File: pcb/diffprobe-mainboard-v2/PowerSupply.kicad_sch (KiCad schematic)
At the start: 19 parts, among them J54 AC_P, J55 AC_N, J56 AC_E

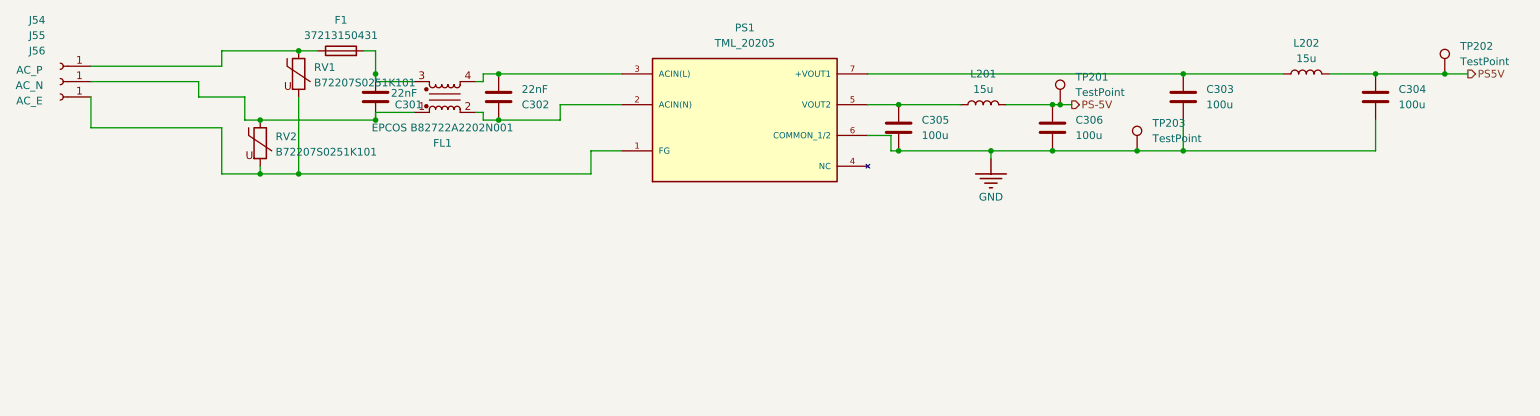
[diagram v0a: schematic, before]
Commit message: schematic cleanup again
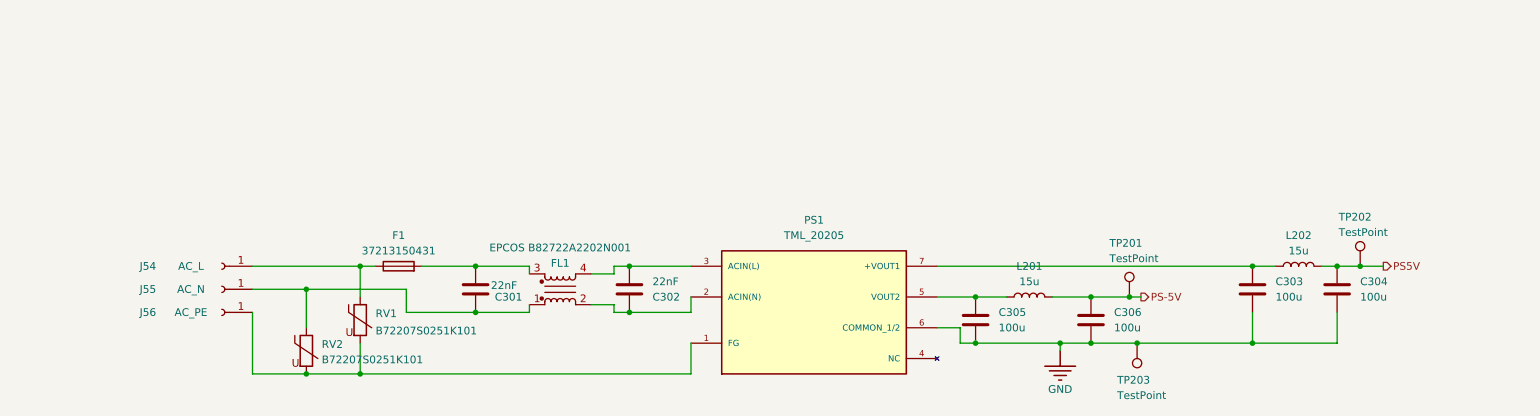
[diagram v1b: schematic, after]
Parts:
- J54: value AC_P -> AC_L
- J56: value AC_E -> AC_PE
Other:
- moved on the sheet: C301, C302, C303, C304, C305, C306, F1, FL1, J54, J55, J56, L201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
